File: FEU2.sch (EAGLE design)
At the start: 48 parts, among them IC1 LM358N, Q1 8M, Q2 32748

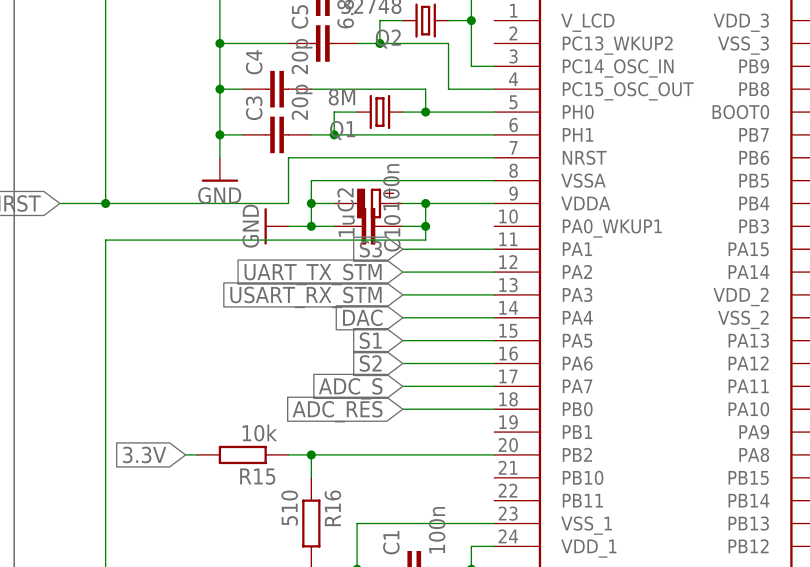
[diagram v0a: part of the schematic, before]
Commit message: BRD 3
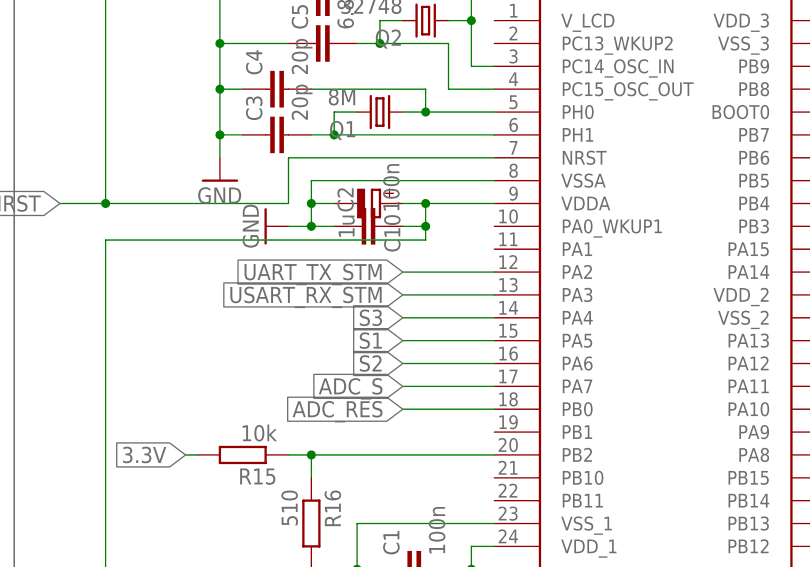
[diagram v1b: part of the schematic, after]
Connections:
- removed net DAC: U$1.PA4
- net S3: now also U$1.PA4; no longer U$1.PA1
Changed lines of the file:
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@@
-</segment>
-</net>
-<net name="DAC" class="0">
-<segment>
-<pinref part="U$1" gate="G$1" pin="PA4"/>
-<wire x1="55.88" y1="58.42" x2="45.72" y2="58.42" width="0.1524" layer="91"/>
-<label x="45.72" y="58.42" size="1.778" layer="95" rot="R180" xref="yes"/>
 </segment>
 </net>
@@
 <net name="S3" class="0">
 <segment>
-<pinref part="U$1" gate="G$1" pin="PA1"/>
-<wire x1="55.88" y1="66.04" x2="45.72" y2="66.04" width="0.1524" layer="91"/>
-<label x="45.72" y="66.04" size="1.778" layer="95" rot="R180" xref="yes"/>
-</segment>
-<segment>
 <pinref part="U$5" gate="G$1" pin="IN1"/>
 <wire x1="88.9" y1="185.42" x2="86.36" y2="185.42" width="0.1524" layer="91"/>
 <label x="86.36" y="185.42" size="1.778" layer="95" rot="R180" xref="yes"/>
 </segment>
+<segment>
+<pinref part="U$1" gate="G$1" pin="PA4"/>
+<wire x1="55.88" y1="58.42" x2="45.72" y2="58.42" width="0.1524" layer="91"/>
+<label x="45.72" y="58.42" size="1.778" layer="95" rot="R180" xref="yes"/>
+</segment>
 </net>
